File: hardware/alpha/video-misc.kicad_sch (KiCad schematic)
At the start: 37 parts, among them J3 SYNC OUT, P30 BANK2_AUX, Q4 BC857, Q5 BC857, Q6 BC807, U1 74LVCH16T245, U3 74LVC1T45, U8 MCP47FEB22A0-E/ST

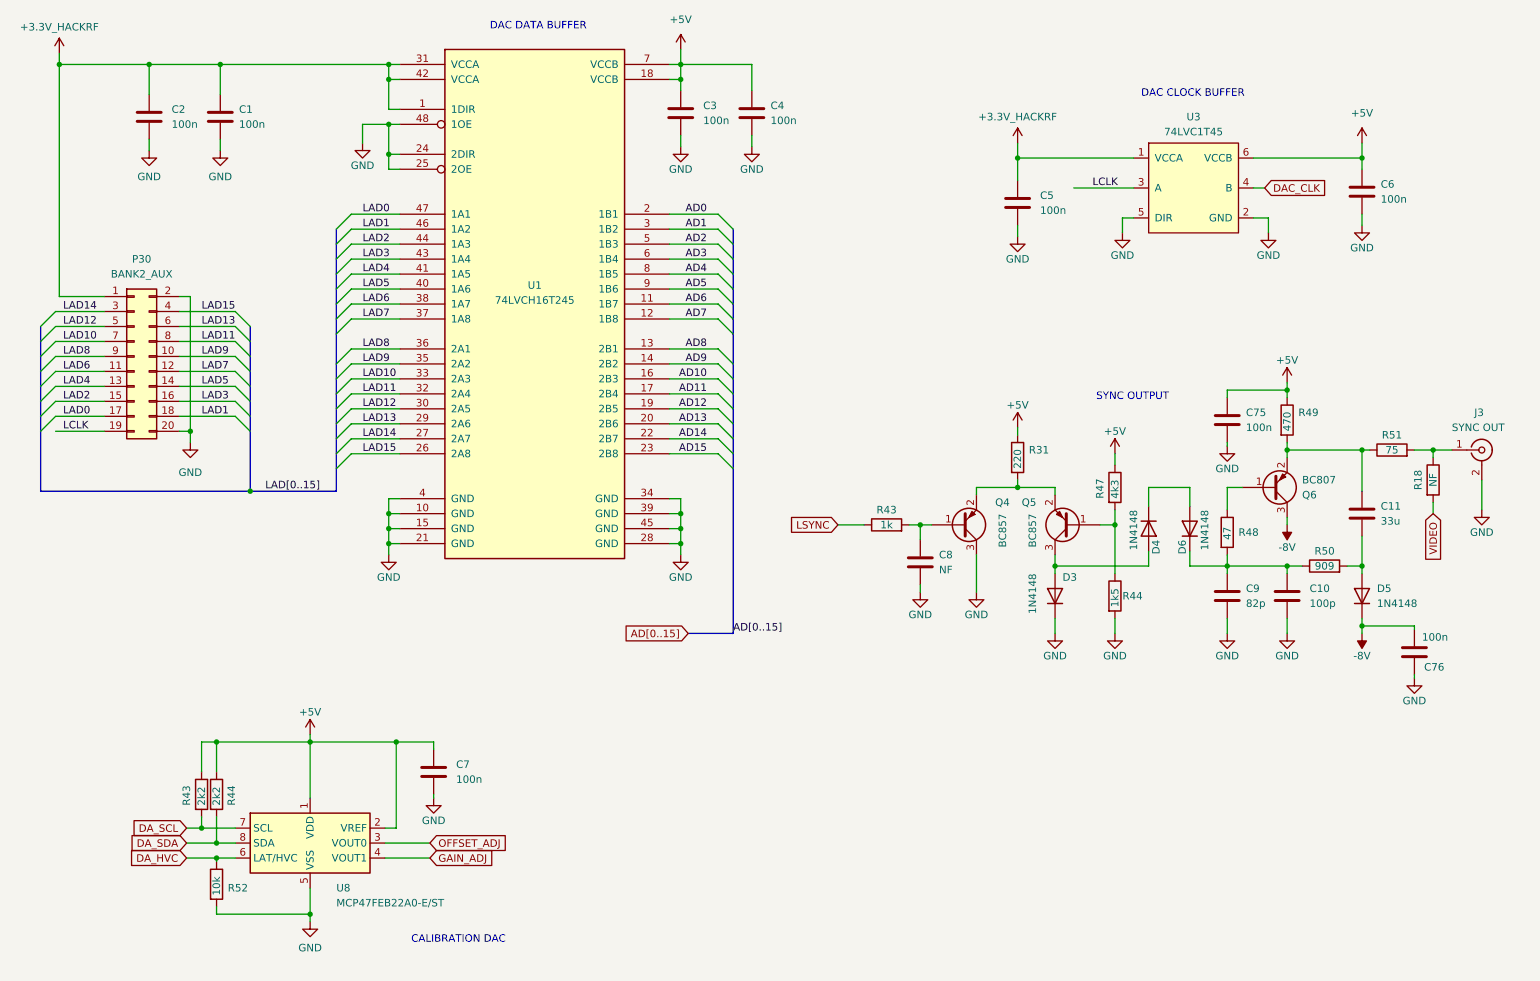
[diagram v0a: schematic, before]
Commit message: WIP
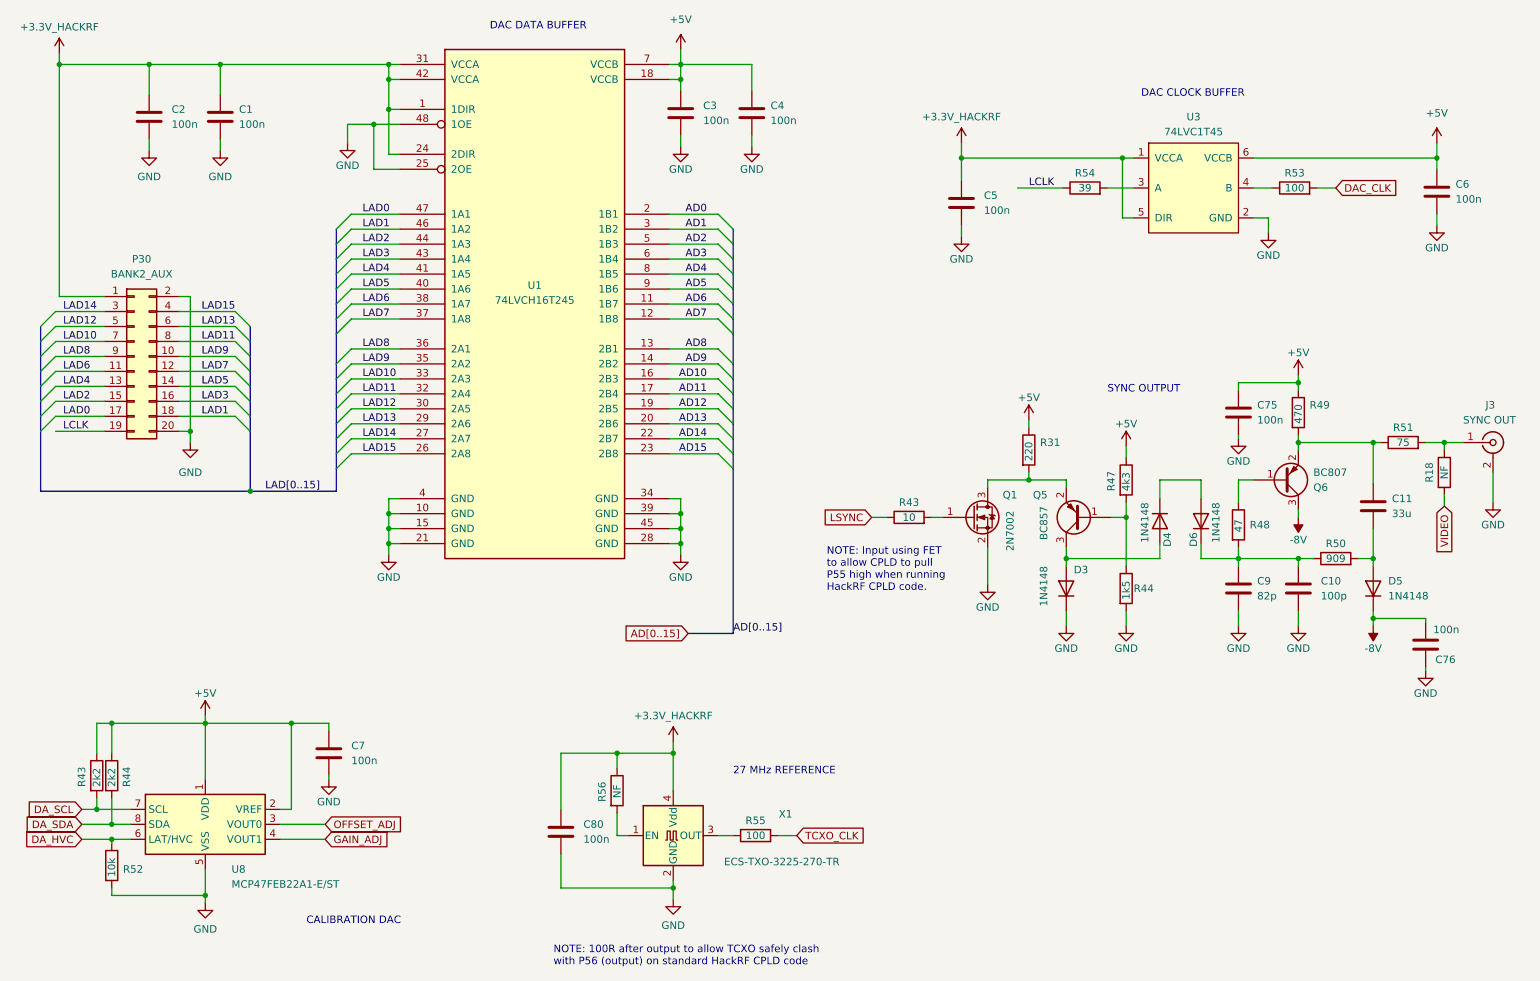
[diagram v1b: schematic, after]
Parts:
- removed C8: NF, Capacitor_SMD:C_0603_1608Metric, symbol Device:C
- removed Q4: BC857, Package_TO_SOT_SMD:SOT-23, symbol Transistor_BJT:BC857
- added C80: 100n, symbol Device:C
- added Q1: 2N7002, Package_TO_SOT_SMD:SOT-23, symbol Transistor_FET:2N7002
- added R53, R55: 100, symbol Device:R
- added R54: 39, symbol Device:R
- added R56: NF, symbol Device:R
- added X1: ECS-TXO-3225-270-TR, Oscillator:Oscillator_SMD_Abracon_ASV-4Pin_7.0x5.1mm, symbol Oscillator:ASV-xxxMHz
- R43: value 1k -> 10
- U8: value MCP47FEB22A0-E/ST -> MCP47FEB22A1-E/ST
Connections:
- net +3.3V_HACKRF: now also U1.24 (2DIR), U3.5 (DIR), C80.1, R56.1, X1.4 (Vdd)
- net DAC_CLK: now also R53.2; no longer U3.4 (B)
- net GND: now also C80.2, Q1.2 (S), X1.2 (GND); no longer U1.24 (2DIR), U3.5 (DIR)
- net LCLK: now also R54.1; no longer U3.3 (A)
- net at R43.2: now also Q1.1 (G)
- net at Q5.2 (E), R31.2: now also Q1.3 (D)
- new net: R56.2, X1.1 (EN)
- new net: R53.1, U3.4 (B)
- new net: R54.2, U3.3 (A)
- new net: R55.1, X1.3 (OUT)
- new net TCXO_CLK: R55.2
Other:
- note added: "27 MHz REFERENCE"
- note added: "NOTE: 100R after output to allow TCXO safely clash with P56 (output) on standard HackRF CPLD code"
- note added: "NOTE: Input using FET to allow CPLD to pull P55 high when running HackRF CPLD code."
- moved on the sheet: C10, C11, C5, C6, C7, C75, C76, C9, D3, D4, D5, D6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
